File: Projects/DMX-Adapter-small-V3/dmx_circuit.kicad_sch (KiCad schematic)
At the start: 5 parts, among them Q2 2N7002, U2 SN75176BDR

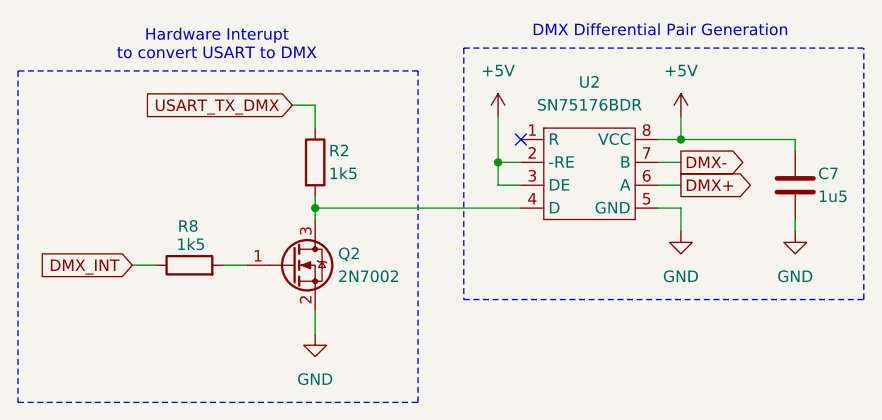
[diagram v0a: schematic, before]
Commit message: preliminary final version
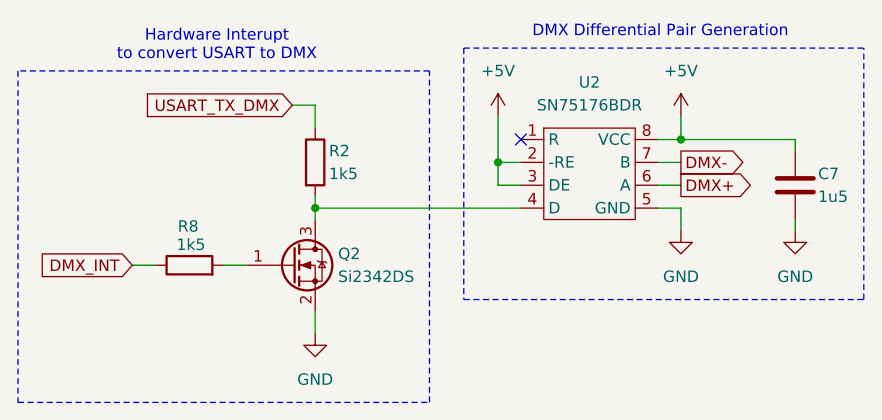
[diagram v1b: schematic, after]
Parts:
- Q2: value 2N7002 -> Si2342DS
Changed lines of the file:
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@@
 	(polyline
 		(pts
-			(xy 101.6 40.64) (xy 57.15 40.64)
+			(xy 102.87 40.64) (xy 57.15 40.64)
 		)
 		(stroke
@@
 	(polyline
 		(pts
-			(xy 101.6 77.47) (xy 101.6 40.64)
+			(xy 102.87 77.47) (xy 102.87 40.64)
 		)
 		(stroke
@@
 	(polyline
 		(pts
-			(xy 57.15 77.47) (xy 101.6 77.47)
+			(xy 57.15 77.47) (xy 102.87 77.47)
 		)
 		(stroke
@@
 			)
 		)
-		(property "Value" "2N7002"
+		(property "Value" "Si2342DS"
 			(at 92.71 63.5 0)
 			(effects
